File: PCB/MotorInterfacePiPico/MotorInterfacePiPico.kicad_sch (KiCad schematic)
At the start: 40 parts, among them J1 Screw_Terminal_01x10, J2 Motor Connector, SW1 SW_DIP_x01, U1 Pico, U2 ILD217T, U3 ILD217T, U4 ILD217T, U5 OPA4197

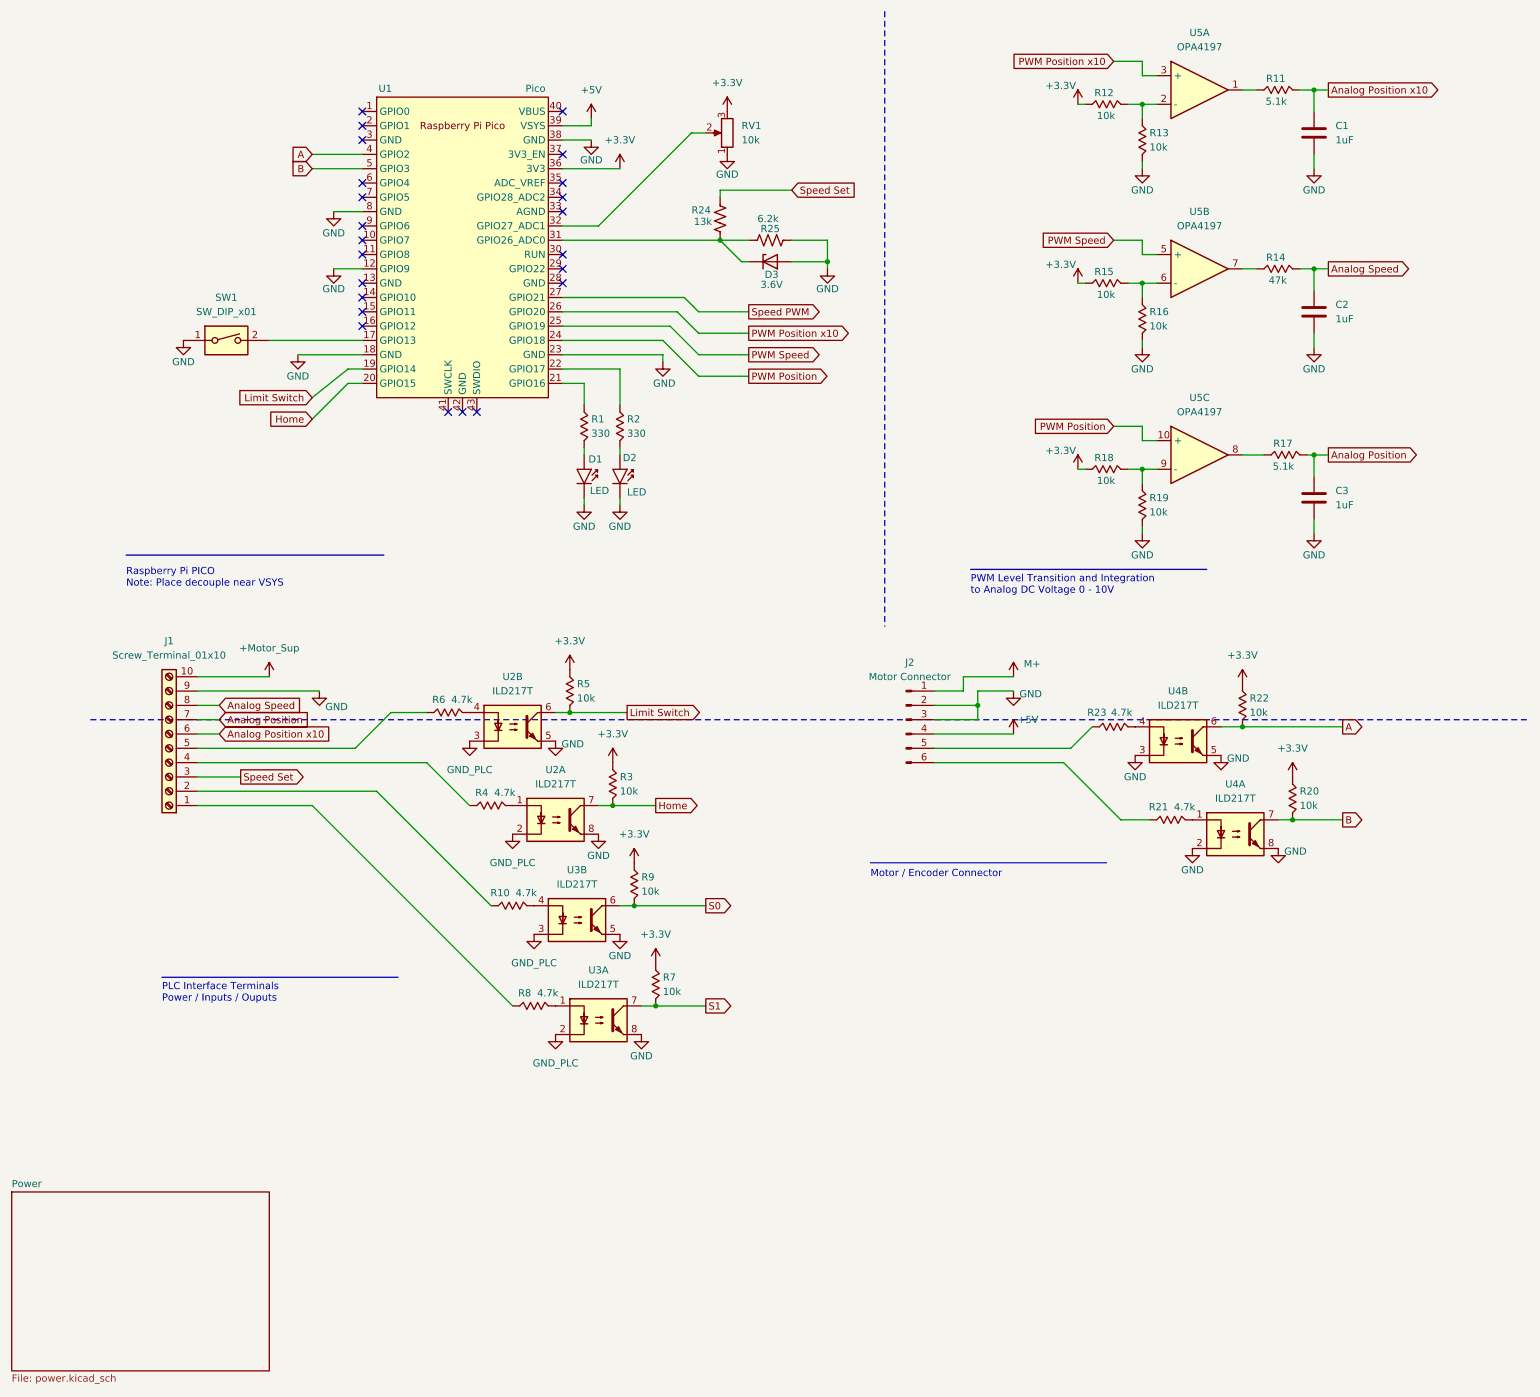
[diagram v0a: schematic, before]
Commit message: Made new Anderson PCB project and reverted Tim R's folder
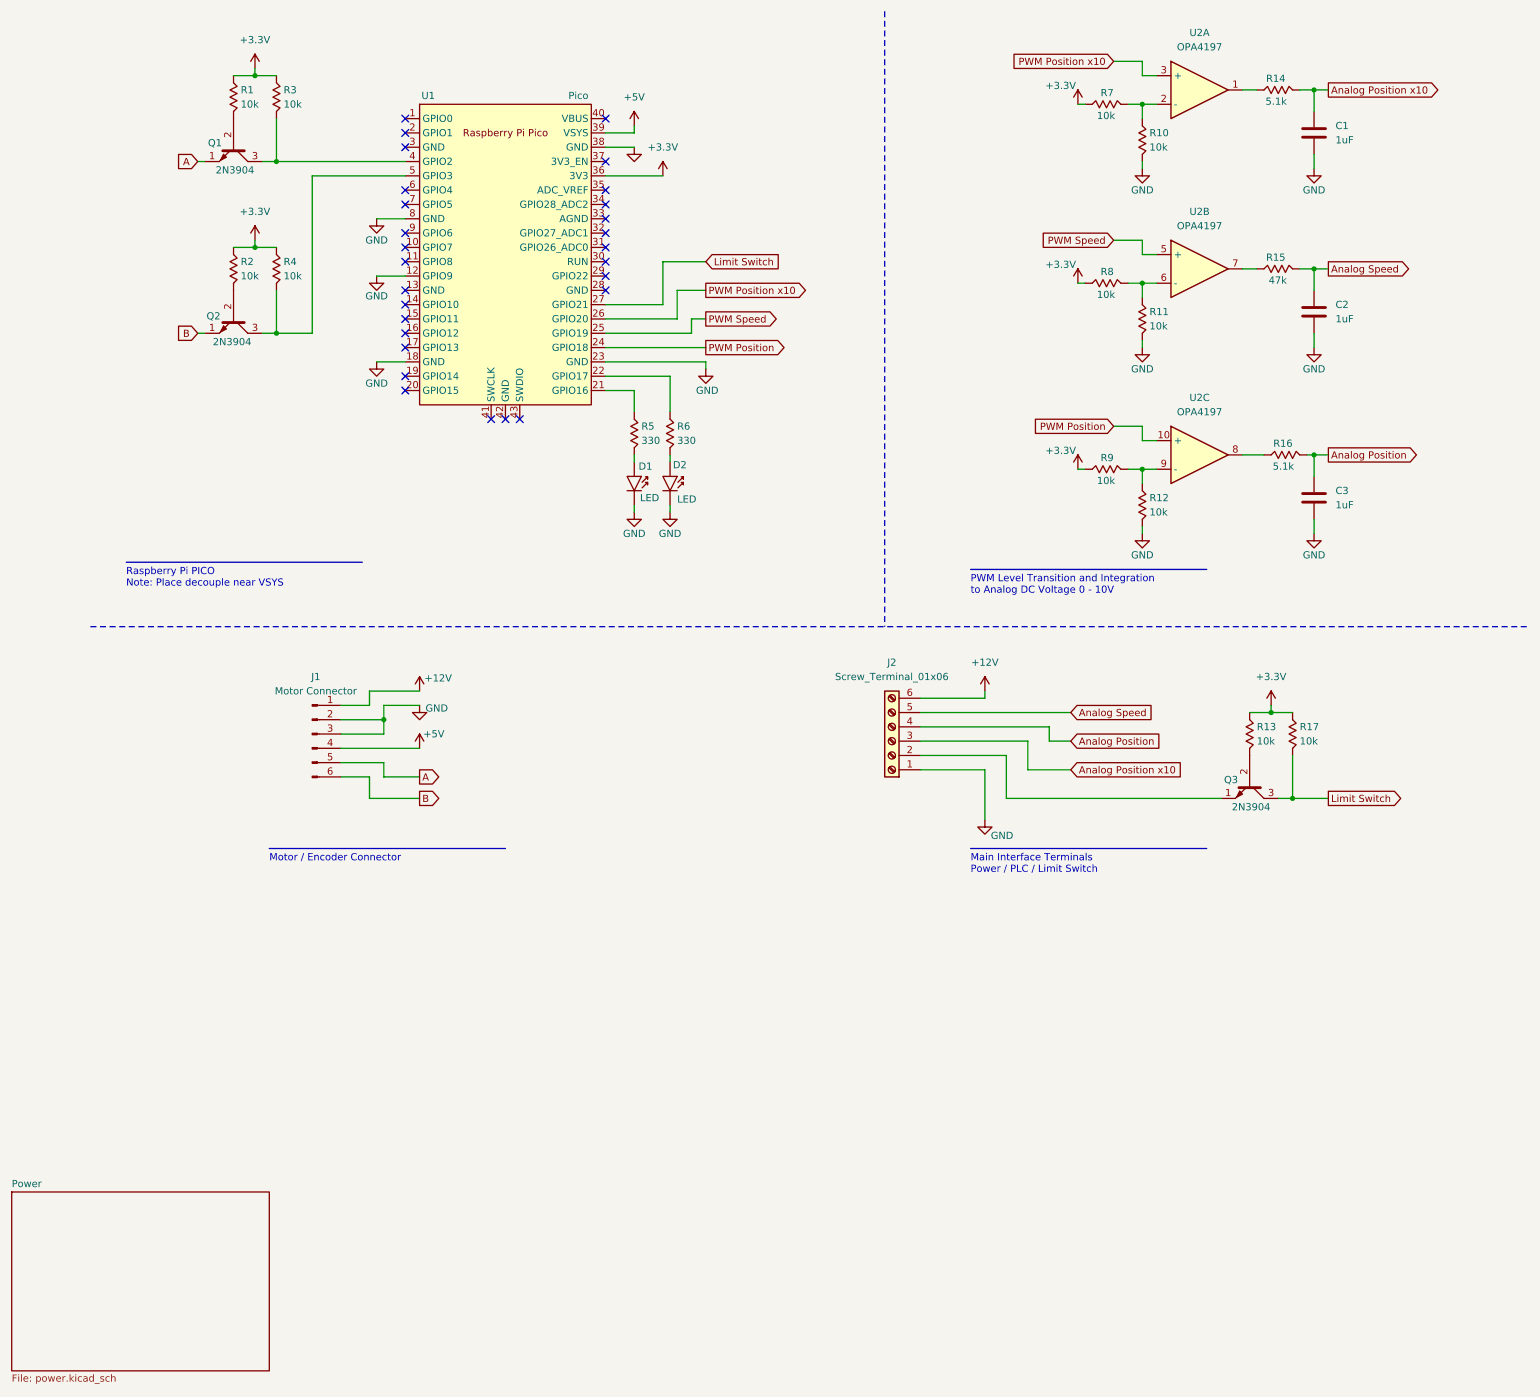
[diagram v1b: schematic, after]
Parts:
- removed D3: 3.6V, Diode_SMD:D_SMA, symbol Diode:Z1SMAxxx
- removed R10, R4, R6, R8: 4.7k, Resistor_SMD:R_0201_0603Metric, symbol TJR:R
- removed R22, R5, R7, R9: 10k, Resistor_SMD:R_0201_0603Metric, symbol TJR:R
- removed R24: 6.2k, Resistor_SMD:R_0201_0603Metric, symbol Device:R_US
- removed R25: 13k, Resistor_SMD:R_0201_0603Metric, symbol Device:R_US
- removed RV1: 10k, Potentiometer_SMD:Potentiometer_ACP_CA6-VSMD_Vertical, symbol Device:R_Potentiometer
- removed SW1: SW_DIP_x01, Button_Switch_SMD:SW_DIP_SPSTx01_Slide_6.7x4.1mm_W8.61mm_P2.54mm_LowProfile, symbol Switch:SW_DIP_x01
- removed U2, U3, U4: ILD217T, CustomBPA:SOIC-8_5.46mm_P1.27, symbol CustomBPA:ILD217T
- added Q1, Q2, Q3: 2N3904, TJR:TO-92-3_Formed_Leads, symbol TJR:2N3904
- added R13, R17: 10k, TJR:R_Axial_DIN0207_L6.3mm_D2.5mm_P7.62mm_Horizontal, symbol TJR:R
- J2: renamed from J1; value Screw_Terminal_01x10 -> Screw_Terminal_01x06; footprint TerminalBlock_Phoenix:TerminalBlock_Phoenix_PT-1,5-10-5.0-H_1x10_P5.00mm_Horizontal -> TerminalBlock_Phoenix:TerminalBlock_Phoenix_PT-1,5-6-5.0-H_1x06_P5.00mm_Horizontal; symbol Connector:Screw_Terminal_01x10 -> Connector:Screw_Terminal_01x06
- R1: renamed from R23; value 4.7k -> 10k; footprint Resistor_SMD:R_0201_0603Metric -> TJR:R_Axial_DIN0207_L6.3mm_D2.5mm_P7.62mm_Horizontal
- R10: renamed from R13; footprint Resistor_SMD:R_0201_0603Metric -> TJR:R_Axial_DIN0207_L6.3mm_D2.5mm_P7.62mm_Horizontal
- R11: renamed from R16; footprint Resistor_SMD:R_0201_0603Metric -> TJR:R_Axial_DIN0207_L6.3mm_D2.5mm_P7.62mm_Horizontal
- R12: renamed from R19; footprint Resistor_SMD:R_0201_0603Metric -> TJR:R_Axial_DIN0207_L6.3mm_D2.5mm_P7.62mm_Horizontal
- R14: renamed from R11; footprint Resistor_SMD:R_0201_0603Metric -> TJR:R_Axial_DIN0207_L6.3mm_D2.5mm_P7.62mm_Horizontal
- R15: renamed from R14; footprint Resistor_SMD:R_0201_0603Metric -> TJR:R_Axial_DIN0207_L6.3mm_D2.5mm_P7.62mm_Horizontal
- R16: renamed from R17; footprint Resistor_SMD:R_0201_0603Metric -> TJR:R_Axial_DIN0207_L6.3mm_D2.5mm_P7.62mm_Horizontal
- R2: renamed from R21; value 4.7k -> 10k; footprint Resistor_SMD:R_0201_0603Metric -> TJR:R_Axial_DIN0207_L6.3mm_D2.5mm_P7.62mm_Horizontal
- R3: footprint Resistor_SMD:R_0201_0603Metric -> TJR:R_Axial_DIN0207_L6.3mm_D2.5mm_P7.62mm_Horizontal
- R4: renamed from R20; footprint Resistor_SMD:R_0201_0603Metric -> TJR:R_Axial_DIN0207_L6.3mm_D2.5mm_P7.62mm_Horizontal
- R5: renamed from R1; footprint Resistor_SMD:R_0201_0603Metric -> TJR:R_Axial_DIN0207_L6.3mm_D2.5mm_P7.62mm_Horizontal
- R6: renamed from R2; footprint Resistor_SMD:R_0201_0603Metric -> TJR:R_Axial_DIN0207_L6.3mm_D2.5mm_P7.62mm_Horizontal
- R7: renamed from R12; footprint Resistor_SMD:R_0201_0603Metric -> TJR:R_Axial_DIN0207_L6.3mm_D2.5mm_P7.62mm_Horizontal
- R8: renamed from R15; footprint Resistor_SMD:R_0201_0603Metric -> TJR:R_Axial_DIN0207_L6.3mm_D2.5mm_P7.62mm_Horizontal
- R9: renamed from R18; footprint Resistor_SMD:R_0201_0603Metric -> TJR:R_Axial_DIN0207_L6.3mm_D2.5mm_P7.62mm_Horizontal
- U2: renamed from U5; footprint CustomBPA:SO-14_5.4_P1.27 -> TJR:D14_TEX
- renumbered J2 to J1
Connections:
- net Speed PWM is gone; now on net Limit Switch: U1.27 (GPIO21)
- net Speed Set is gone; now on net Analog Position x10: J2.3 (Pin_3)
- net +3.3V: now also R1.1, R2.1, R13.1, R17.1
- net A: now also J1.5 (Pin_5), Q1.1 (E); no longer U1.4 (GPIO2)
- net Analog Position: now also J2.4 (Pin_4); no longer J2.7 (Pin_7)
- net Analog Position x10: no longer J2.6 (Pin_6)
- net Analog Speed: now also J2.5 (Pin_5); no longer J2.8 (Pin_8)
- net B: now also J1.6 (Pin_6), Q2.1 (E); no longer R4.2, U1.5 (GPIO3)
- net GND: now also J2.1 (Pin_1); no longer J2.9 (Pin_9)
- net Limit Switch: now also Q3.3 (C), R17.2; no longer U1.19 (GPIO14)
- net at J2.2 (Pin_2): now also Q3.1 (E)
- net at R2.2: now also Q2.2 (B)
- net at R1.2: now also Q1.2 (B)
- removed net +Motor_Sup: J2.10 (Pin_10)
- net Home: no longer names the net of U1.20 (GPIO15)
- net Home: no longer R3.2
- net M+ renamed +12V
- net +12V: now also J2.6 (Pin_6)
- new net: Q1.3 (C), R3.2, U1.4 (GPIO2)
- new net: Q2.3 (C), R4.2, U1.5 (GPIO3)
- new net: Q3.2 (B), R13.2
- no-connect marks 23 -> 28
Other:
- note added: "Main Interface Terminals Power / PLC / Limit Switch"
- note removed: "PLC Interface Terminals Power / Inputs / Ouputs"
- moved on the sheet: D1, D2, J1, R1, R2, R4, R5, R6, U1

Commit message: Surface Mount Board design
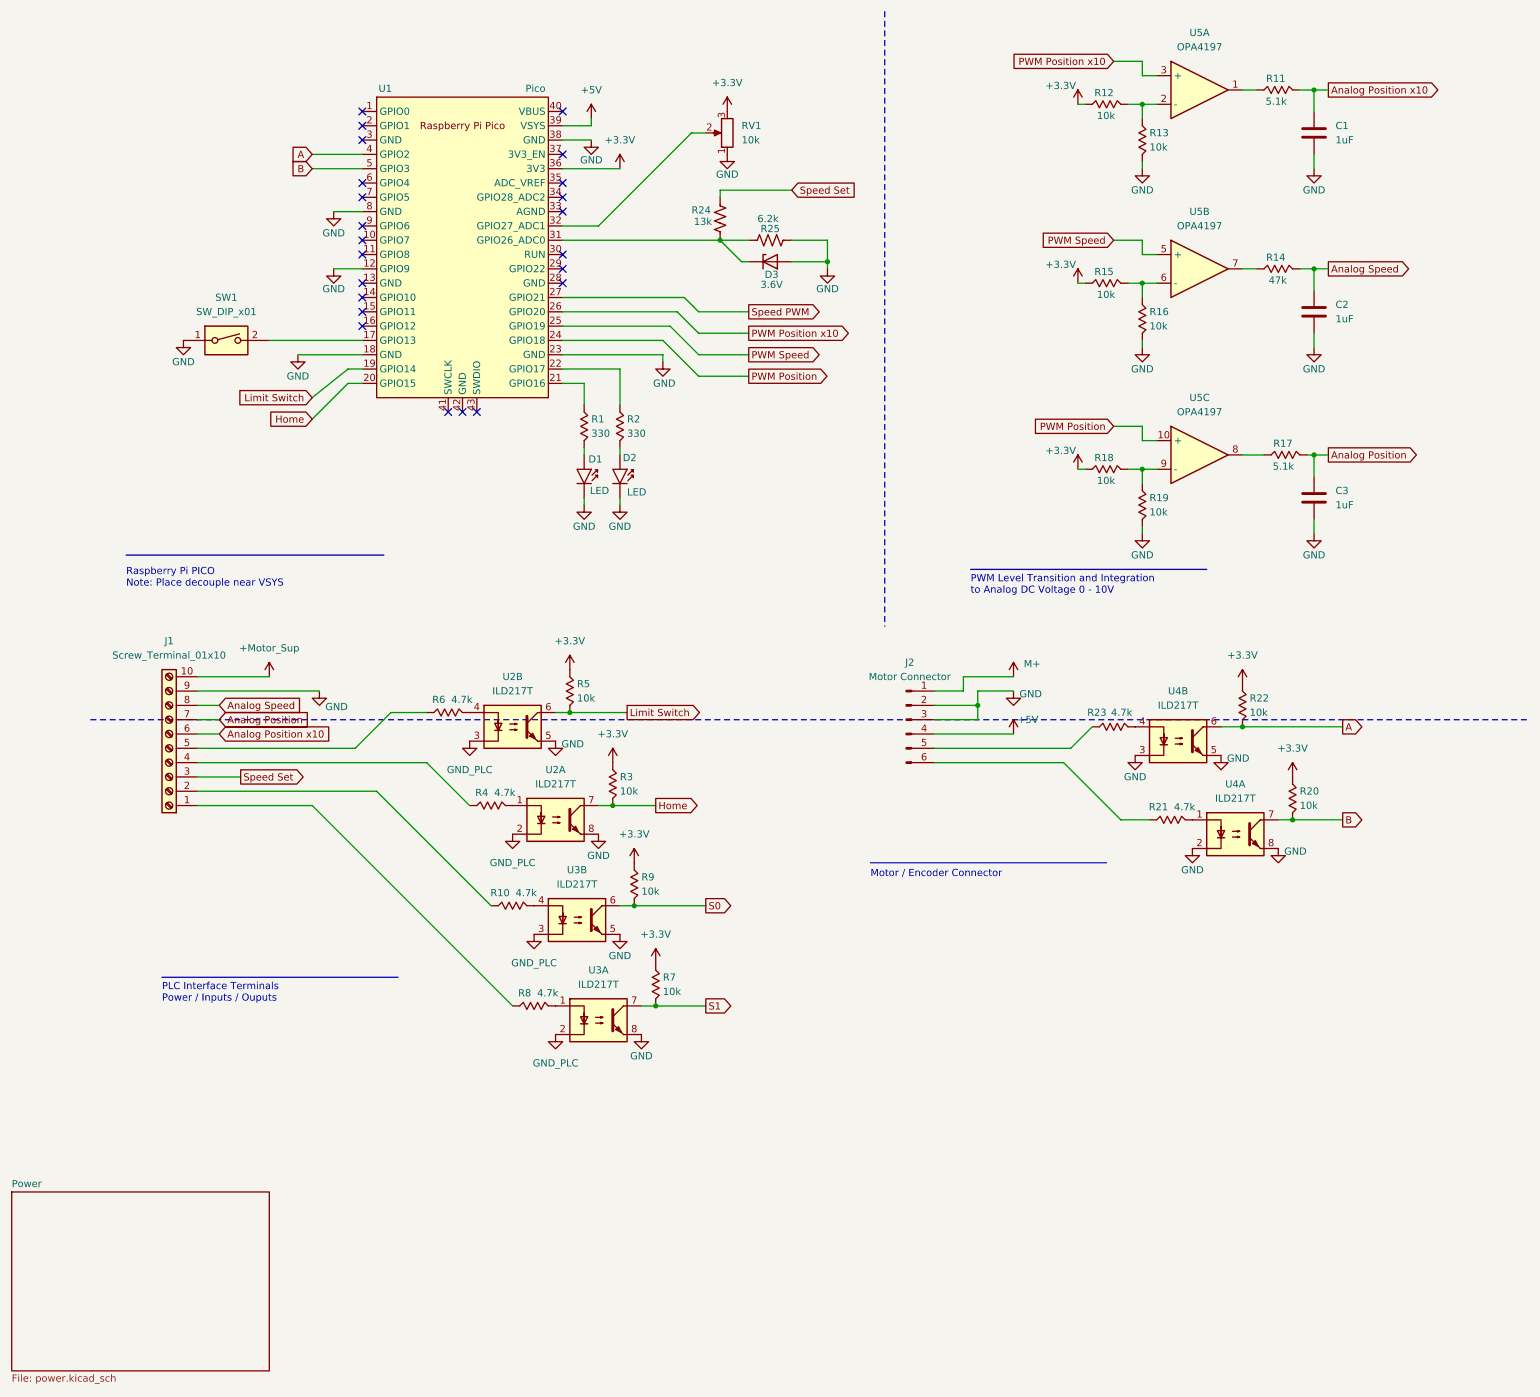
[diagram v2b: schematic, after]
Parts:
- removed Q1, Q2, Q3: 2N3904, TJR:TO-92-3_Formed_Leads, symbol TJR:2N3904
- removed R13, R17: 10k, TJR:R_Axial_DIN0207_L6.3mm_D2.5mm_P7.62mm_Horizontal, symbol TJR:R
- added D3: 3.6V, Diode_SMD:D_SMA, symbol Diode:Z1SMAxxx
- added R10, R4, R6, R8: 4.7k, Resistor_SMD:R_0201_0603Metric, symbol TJR:R
- added R22, R5, R7, R9: 10k, Resistor_SMD:R_0201_0603Metric, symbol TJR:R
- added R24: 6.2k, Resistor_SMD:R_0201_0603Metric, symbol Device:R_US
- added R25: 13k, Resistor_SMD:R_0201_0603Metric, symbol Device:R_US
- added RV1: 10k, Potentiometer_SMD:Potentiometer_ACP_CA6-VSMD_Vertical, symbol Device:R_Potentiometer
- added SW1: SW_DIP_x01, Button_Switch_SMD:SW_DIP_SPSTx01_Slide_6.7x4.1mm_W8.61mm_P2.54mm_LowProfile, symbol Switch:SW_DIP_x01
- added U2, U3, U4: ILD217T, CustomBPA:SOIC-8_5.46mm_P1.27, symbol CustomBPA:ILD217T
- J1: renamed from J2; value Screw_Terminal_01x06 -> Screw_Terminal_01x10; footprint TerminalBlock_Phoenix:TerminalBlock_Phoenix_PT-1,5-6-5.0-H_1x06_P5.00mm_Horizontal -> TerminalBlock_Phoenix:TerminalBlock_Phoenix_PT-1,5-10-5.0-H_1x10_P5.00mm_Horizontal; symbol Connector:Screw_Terminal_01x06 -> Connector:Screw_Terminal_01x10
- R1: renamed from R5; footprint TJR:R_Axial_DIN0207_L6.3mm_D2.5mm_P7.62mm_Horizontal -> Resistor_SMD:R_0201_0603Metric
- R11: renamed from R14; footprint TJR:R_Axial_DIN0207_L6.3mm_D2.5mm_P7.62mm_Horizontal -> Resistor_SMD:R_0201_0603Metric
- R12: renamed from R7; footprint TJR:R_Axial_DIN0207_L6.3mm_D2.5mm_P7.62mm_Horizontal -> Resistor_SMD:R_0201_0603Metric
- R13: renamed from R10; footprint TJR:R_Axial_DIN0207_L6.3mm_D2.5mm_P7.62mm_Horizontal -> Resistor_SMD:R_0201_0603Metric
- R14: renamed from R15; footprint TJR:R_Axial_DIN0207_L6.3mm_D2.5mm_P7.62mm_Horizontal -> Resistor_SMD:R_0201_0603Metric
- R15: renamed from R8; footprint TJR:R_Axial_DIN0207_L6.3mm_D2.5mm_P7.62mm_Horizontal -> Resistor_SMD:R_0201_0603Metric
- R16: renamed from R11; footprint TJR:R_Axial_DIN0207_L6.3mm_D2.5mm_P7.62mm_Horizontal -> Resistor_SMD:R_0201_0603Metric
- R17: renamed from R16; footprint TJR:R_Axial_DIN0207_L6.3mm_D2.5mm_P7.62mm_Horizontal -> Resistor_SMD:R_0201_0603Metric
- R18: renamed from R9; footprint TJR:R_Axial_DIN0207_L6.3mm_D2.5mm_P7.62mm_Horizontal -> Resistor_SMD:R_0201_0603Metric
- R19: renamed from R12; footprint TJR:R_Axial_DIN0207_L6.3mm_D2.5mm_P7.62mm_Horizontal -> Resistor_SMD:R_0201_0603Metric
- R2: renamed from R6; footprint TJR:R_Axial_DIN0207_L6.3mm_D2.5mm_P7.62mm_Horizontal -> Resistor_SMD:R_0201_0603Metric
- R20: renamed from R4; footprint TJR:R_Axial_DIN0207_L6.3mm_D2.5mm_P7.62mm_Horizontal -> Resistor_SMD:R_0201_0603Metric
- R21: renamed from R2; value 10k -> 4.7k; footprint TJR:R_Axial_DIN0207_L6.3mm_D2.5mm_P7.62mm_Horizontal -> Resistor_SMD:R_0201_0603Metric
- R23: renamed from R1; value 10k -> 4.7k; footprint TJR:R_Axial_DIN0207_L6.3mm_D2.5mm_P7.62mm_Horizontal -> Resistor_SMD:R_0201_0603Metric
- R3: footprint TJR:R_Axial_DIN0207_L6.3mm_D2.5mm_P7.62mm_Horizontal -> Resistor_SMD:R_0201_0603Metric
- U5: renamed from U2; footprint TJR:D14_TEX -> CustomBPA:SO-14_5.4_P1.27
- renumbered J1 to J2
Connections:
- net +3.3V: now also R22.1, R5.1, R7.1, R9.1, RV1.3; no longer R21.1, R23.1
- net A: now also U1.4 (GPIO2), R22.2, U4.6; no longer J2.5 (Pin_5)
- net Analog Position: now also J1.7 (Pin_7); no longer J1.4 (Pin_4)
- net Analog Position x10: now also J1.6 (Pin_6); no longer J1.3 (Pin_3)
- net Analog Speed: now also J1.8 (Pin_8); no longer J1.5 (Pin_5)
- net B: now also R20.2, U1.5 (GPIO3), U4.7; no longer J2.6 (Pin_6)
- net GND: now also J1.9 (Pin_9), D3.2 (A), R25.1, RV1.1, SW1.1, U2.5, U2.8, U3.5, U3.8, U4.2, U4.3, U4.5, U4.8; no longer J1.1 (Pin_1)
- net Limit Switch: now also U1.19 (GPIO14), R5.2, U2.6; no longer U1.27 (GPIO21)
- net at J1.2 (Pin_2): now also R10.1
- net at U1.17 (GPIO13): now also SW1.2
- net Home: now reaches U1.20 (GPIO15)
- net Home: now also R3.2, U2.7
- net at U1.31 (GPIO26_ADC0): now also D3.1 (K), R24.2, R25.2
- net at U1.32 (GPIO27_ADC1): now also RV1.2
- net at R23.2: now also U4.4
- net at R21.2: now also U4.1
- net +12V renamed M+
- net M+: no longer J1.6 (Pin_6)
- new net: J1.1 (Pin_1), R8.1
- new net: J1.4 (Pin_4), R4.1
- new net: J1.5 (Pin_5), R6.1
- new net: R10.2, U3.4
- new net: J2.5 (Pin_5), R23.1
- new net: R4.2, U2.1
- new net: R6.2, U2.4
- new net: R8.2, U3.1
- new net: J2.6 (Pin_6), R21.1
- new net +Motor_Sup: J1.10 (Pin_10)
- new net GND_PLC: U2.2, U2.3, U3.2, U3.3
- new net S0: R9.2, U3.6
- new net S1: R7.2, U3.7
- new net Speed PWM: U1.27 (GPIO21)
- new net Speed Set: J1.3 (Pin_3), R24.1
- no-connect marks 28 -> 23
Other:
- note added: "PLC Interface Terminals Power / Inputs / Ouputs"
- note removed: "Main Interface Terminals Power / PLC / Limit Switch"
- moved on the sheet: D1, D2, J2, R1, R2, R20, R21, R23, U1
